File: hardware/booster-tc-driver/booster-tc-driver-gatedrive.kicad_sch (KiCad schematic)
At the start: 34 parts, among them IC6 SI4564DY-T1-GE3, IC7 SI4564DY-T1-GE3, IC8 SI4564DY-T1-GE3, IC9 SI4564DY-T1-GE3, J4 22-23-2021, J5 22-23-2021, U8 UCC21520DW, U9 UCC21520DW

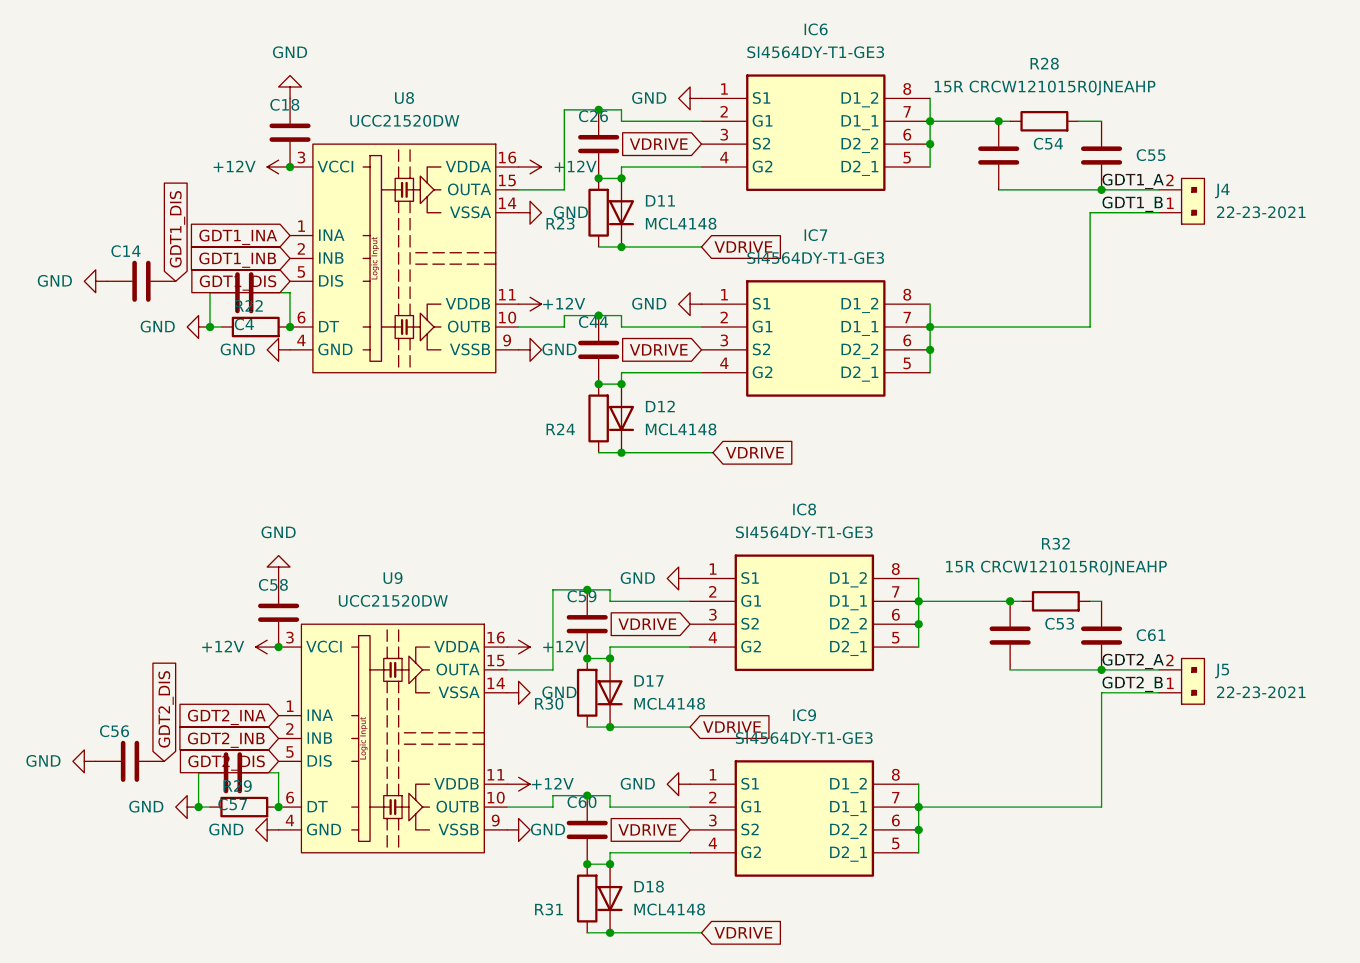
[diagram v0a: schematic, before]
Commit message: schematic cleanup
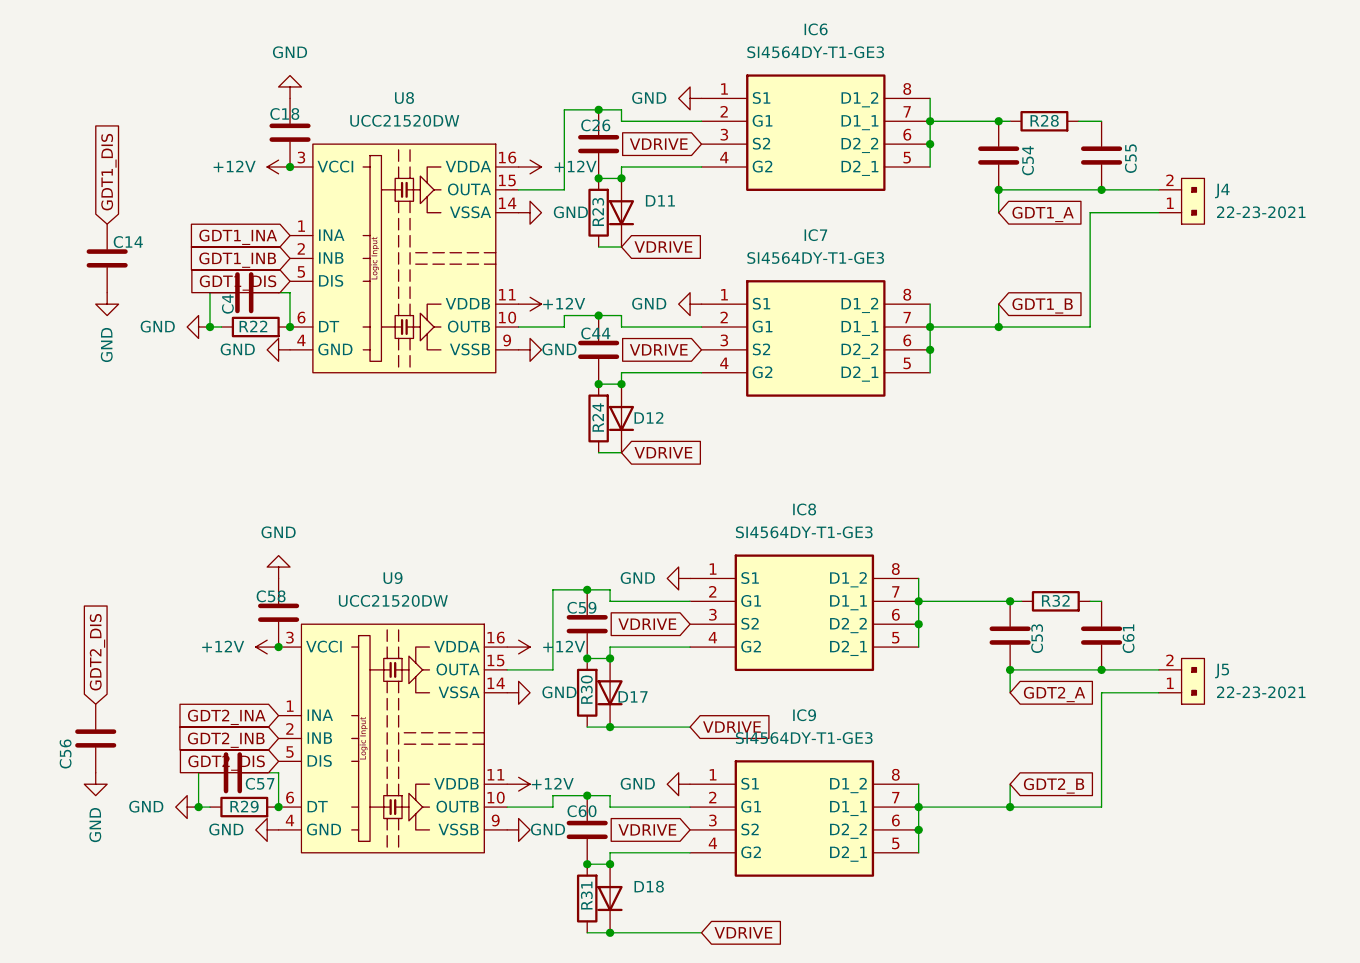
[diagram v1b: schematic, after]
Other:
- moved on the sheet: C14, C56

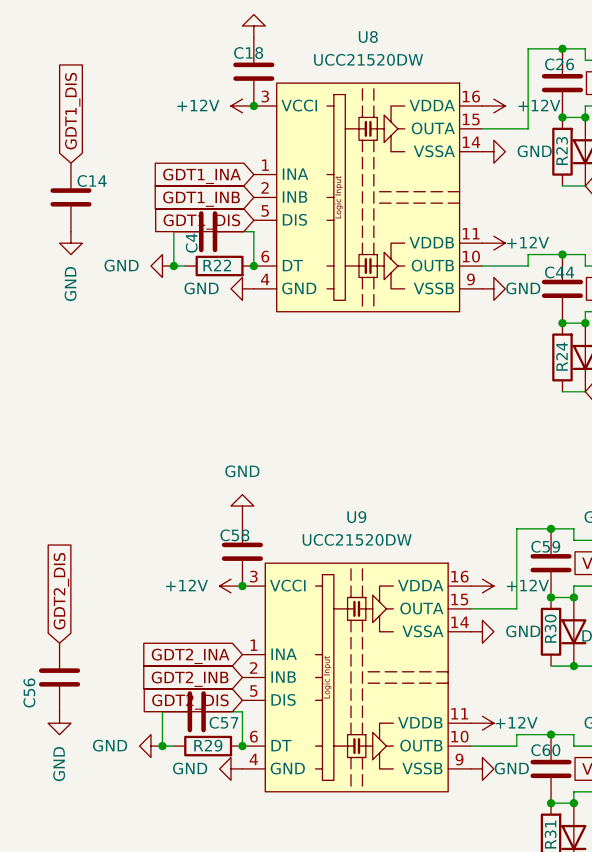
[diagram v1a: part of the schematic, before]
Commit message: changed pin assignments, improved hardware
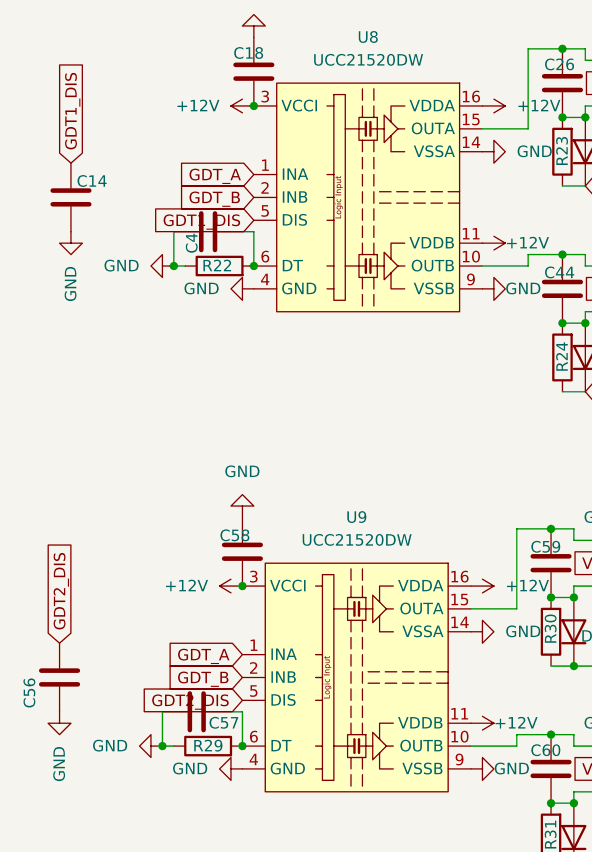
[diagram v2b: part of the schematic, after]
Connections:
- net GDT2_INA is gone; now on net GDT_A: U9.1 (INA)
- net GDT2_INB is gone; now on net GDT_B: U9.2 (INB)
- net GDT1_INA renamed GDT_A
- net GDT1_INB renamed GDT_B
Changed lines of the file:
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@@
 		)
 	)
-	(global_label "GDT2_INB"
+	(global_label "GDT_B"
 		(shape input)
 		(at 91.44 101.6 180)
@@
 		)
 		(property "Intersheetrefs" "${INTERSHEET_REFS}"
-			(at 79.5648 101.6 0)
+			(at 82.7096 101.6 0)
 			(effects
 				(font
@@
 		)
 	)
-	(global_label "GDT2_INA"
+	(global_label "GDT_A"
 		(shape input)
 		(at 91.44 99.06 180)
@@
 		)
 		(property "Intersheetrefs" "${INTERSHEET_REFS}"
-			(at 79.7462 99.06 0)
+			(at 82.891 99.06 0)
 			(effects
 				(font
@@
 		)
 	)
-	(global_label "GDT1_INB"
+	(global_label "GDT_B"
 		(shape input)
 		(at 92.71 48.26 180)
@@
 		)
 		(property "Intersheetrefs" "${INTERSHEET_REFS}"
-			(at 80.8348 48.26 0)
+			(at 83.9796 48.26 0)
 			(effects
 				(font
@@
 		)
 	)
-	(global_label "GDT1_INA"
+	(global_label "GDT_A"
 		(shape input)
 		(at 92.71 45.72 180)
@@
 		)
 		(property "Intersheetrefs" "${INTERSHEET_REFS}"
-			(at 81.0162 45.72 0)
-			(effects
-				(font
+			(at 84.161 45.72 0)
+			(effects
+				(font
